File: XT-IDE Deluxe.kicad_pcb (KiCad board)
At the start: 2 copper layers, 100.4 x 96 mm, 58 parts, among them J1 IDE, J10 IRQ5, J11 IRQ7, J2 CF_Adapter, J3 IDE IRQ, J4 VCC, J5 Power Output, J6 MemExp, J7 IRQ2, J8 IRQ3, J9 IRQ4, SW1 HiSpeed, SW2 Config, U1 HCT245, U10 F138, U12 HCT02, U13 AHC1G09, U14 F138, U15 HCT86, U16 F138, U2 HCT573, U3 HCT573, U4 HCT245, U5 HCT04, U6 HCT32, U7 HCT04, U8 28C256, U9 HCT86

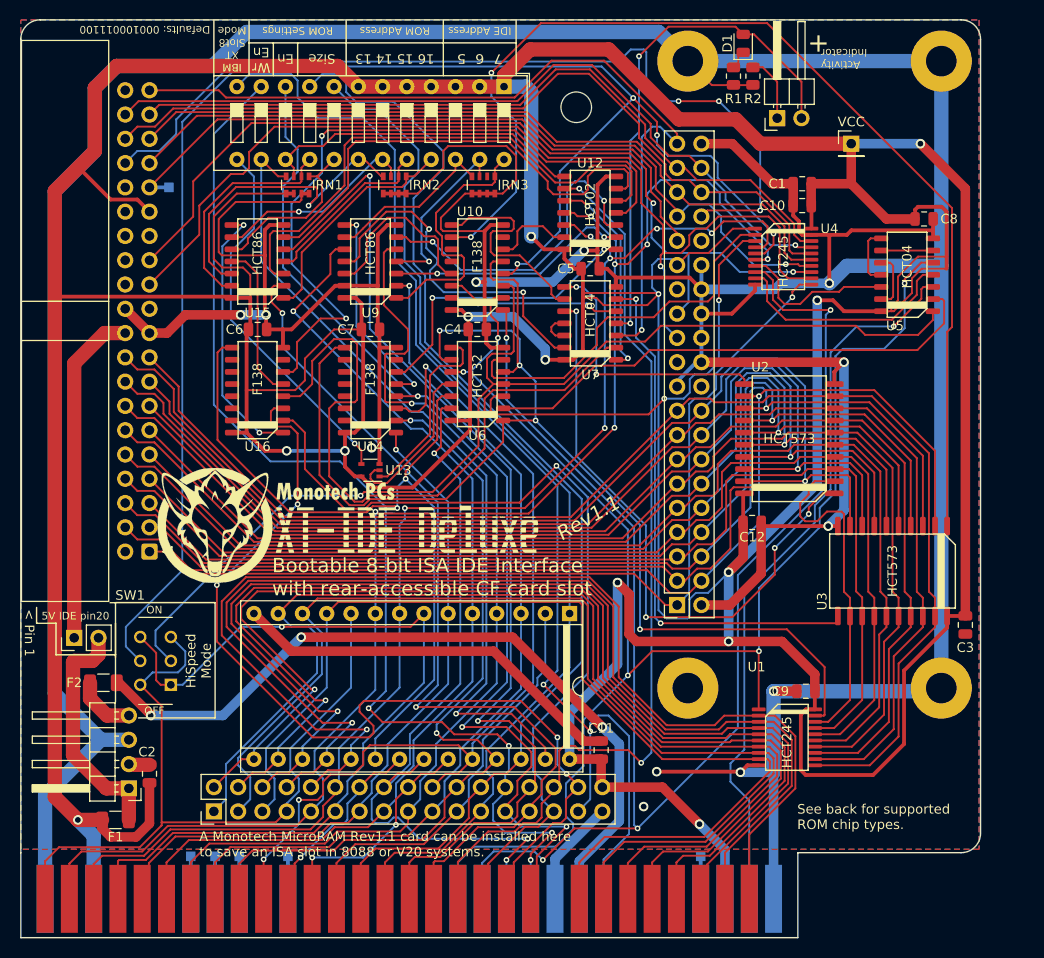
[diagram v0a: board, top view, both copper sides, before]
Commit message: Update to v1.2.
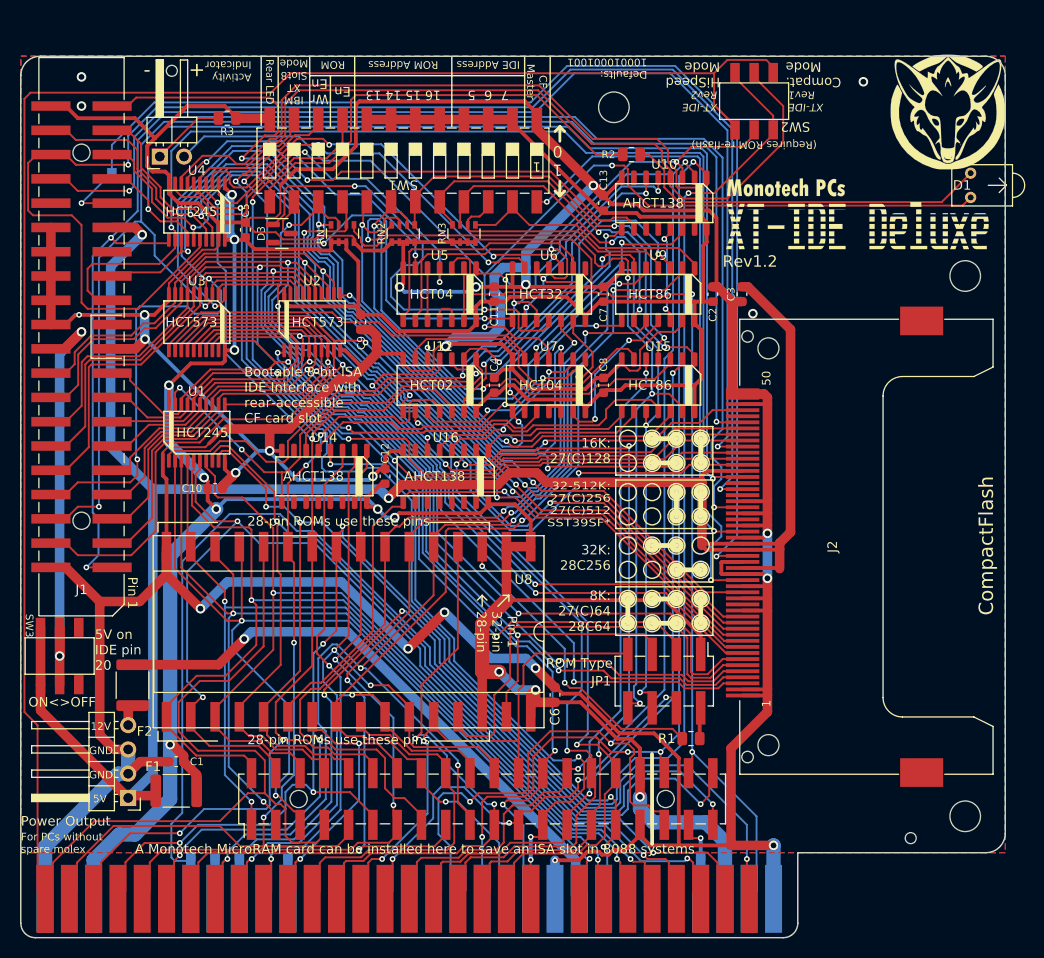
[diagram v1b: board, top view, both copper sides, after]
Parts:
- removed H3, H4: M3, MountingHole:MountingHole_3.2mm_M3_Pad
- removed H5: MountingHole, MountingHole:MountingHole_3.2mm_M3
- removed J4: VCC, Connector_PinHeader_2.54mm:PinHeader_1x01_P2.54mm_Vertical
- removed U13: AHC1G09, Package_TO_SOT_SMD:SOT-353_SC-70-5
- added C13: 100nF, Capacitor_SMD:C_0603_1608Metric, F.Cu at (224.6, 38.6)
- added D3: BAT54A, Package_TO_SOT_SMD:SOT-23, F.Cu at (190.9, 41.8)
- added R3: 220, Resistor_SMD:R_0805_2012Metric, F.Cu at (185.2, 29.7)
- added REF**: JLC_Tooling_Hole, Custom KiCad Library:JLC_Tooling_Hole, F.Cu at (179.4, 24.7)
- added REF**: JLC_Tooling_Hole, Custom KiCad Library:JLC_Tooling_Hole, F.Cu at (256.7, 105.0)
- added SW3: 5V on IDE Pin20, Custom:SW_DPDT_MS-22D28-G020, F.Cu at (167.7, 86.0)
- BUS1: value Bus_ISA_8bit -> 8-bit ISA
- C1, C2: value 106 -> 10uF; footprint Capacitor_SMD:C_0805_2012Metric -> Capacitor_SMD:C_0603_1608Metric
- C10, C11, C12, C3, C4, C5, C6, C7, C8, C9: value 104 -> 100nF; footprint Capacitor_SMD:C_0805_2012Metric -> Capacitor_SMD:C_0603_1608Metric
- D1: value LED -> Rear LED; footprint LED_SMD:LED_0805_2012Metric -> Custom:3mm_LED_RightAngle
- D2: value LED -> LED Header
- F1, F2: footprint Fuse:Fuse_1206_3216Metric -> Fuse:Fuse_1812_4532Metric
- H1, H2: value M3 -> MountingHole; footprint MountingHole:MountingHole_3.2mm_M3_Pad -> MountingHole:MountingHole_3.2mm_M3
- J1: footprint Connector_IDC:IDC-Header_2x20_P2.54mm_Horizontal -> Custom:IDC-20_P2.54mm_Vertical_SMD
- J2: value CF_Adapter -> CF Slot; footprint Connector_PinSocket_2.54mm:PinSocket_2x20_P2.54mm_Vertical -> Custom:CF_Slot_UMax_CFH-R3C1LBMXXMN2
- J6: footprint Connector_PinHeader_2.54mm:PinHeader_2x17_P2.54mm_Vertical -> Custom:MicroRAM_Expansion
- JP1: value 5V IDE pin20 -> ROM Type; footprint Connector_PinHeader_2.54mm:PinHeader_1x02_P2.54mm_Vertical -> Custom:PinHeader_2x04_P2.54mm_Vertical_SMD
- R1, R2: value 1k -> 220
- SW1: value HiSpeed -> Config; footprint Monotech Obscure KiCad Library:SW_MS-22D18G2 -> Button_Switch_SMD:SW_DIP_SPSTx12_Slide_6.7x32.04mm_W8.61mm_P2.54mm_LowProfile
- SW2: value Config -> Rev2; footprint Button_Switch_THT:SW_DIP_SPSTx12_Slide_9.78x32.66mm_W7.62mm_P2.54mm -> Custom:SW_DPDT_MS-22D28-G020
- U10, U14, U16: value F138 -> AHCT138
- U2, U3: footprint Custom KiCad Library:SOIC-20W_7.5x12.8mm_P1.27mm -> Custom KiCad Library:TSSOP-20_4.4x6.5mm_P0.65mm
- U8: value 28C256 -> ROM; footprint Custom KiCad Library:DIP-28_W15.24mm_Socket -> Custom:DIP-32_W16.51mm_SMDSocket_LongPads
- moved C1 89.1 mm to (179.9, 97.0)
- moved LOGO1 88.0 mm to (260.6, 29.1)
- moved H2 84.2 mm to (262.4, 102.7)
- moved C2 77.4 mm to (236.0, 48.1)
- moved U3 77.3 mm to (182.0, 51.0)
- moved U1 69.5 mm to (182.0, 62.6), turned to 90 degrees
- moved R1 69.4 mm to (233.7, 94.6), turned to 0 degrees
- moved C10 68.2 mm to (183.9, 68.4), turned to 0 degrees
- moved D2 64.7 mm to (178.2, 33.7)
- moved JP1 61.9 mm to (230.9, 88.6), turned to -90 degrees
- moved U4 61.5 mm to (182.0, 39.5), turned to -90 degrees
- moved C9 60.5 mm to (199.2, 51.0), turned to -90 degrees
- moved SW1 58.4 mm to (203.6, 34.1), turned to -90 degrees
- moved LOGO2 56.8 mm to (251.3, 39.9)
- moved H1 52.0 mm to (262.4, 46.2)
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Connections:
- net /~{LA1-OE} renamed /~{LA1_OE}
- net /~{LA2-OE} renamed /~{LA2_OE}
- net /~{xLA2-OE} renamed /~{xLA2_OE}
- C3 pad 1: VCC -> /5V_Fused
- F1 pad 1: VCC -> /5V_Fused
- F1 pad 2: /5V_Fused -> VCC
- F2 pad 1: +12V -> /12V_Fused
- F2 pad 2: Net-(F2-Pad2) -> +12V
- J1 pad 20: /IDE_5V -> /IDE_pin20
- J1 pad 21: (no net) -> unconnected-(J1-Pad21)
- J1 pad 27: (no net) -> unconnected-(J1-Pad27)
- J1 pad 29: VCC -> /5V_Fused
- J1 pad 32: (no net) -> unconnected-(J1-Pad32)
- J1 pad 35: /BA0-OR-BA3 -> /B_A0_A3
- J2 pad 1: /~{BRST} -> GND
- J2 pad 10: /DB11 -> GND
- J2 pad 11: /DB3 -> GND
- J2 pad 12: /DB12 -> GND
- J2 pad 13: /DB2 -> /5V_Fused
- J2 pad 14: /DB13 -> GND
- J2 pad 15: /DB1 -> GND
- J2 pad 16: /DB14 -> GND
- J2 pad 17: /DB0 -> GND
- J2 pad 18: /DB15 -> /BA2
- J2 pad 19: GND -> /BA1
- J2 pad 2: GND -> /DB3
- J2 pad 20: (no net) -> /B_A0_A3
- J2 pad 21: (no net) -> /DB0
- J2 pad 22: GND -> /DB1
- J2 pad 23: /~{BIOW} -> /DB2
- J2 pad 24: GND -> unconnected-(J2-Pad24)
- J2 pad 25: /~{BIOR} -> GND
- J2 pad 27: (no net) -> /DB11
- J2 pad 28: GND -> /DB12
- J2 pad 29: VCC -> /DB13
- J2 pad 3: /DB7 -> /DB4
- J2 pad 30: GND -> /DB14
- J2 pad 31: /IDE_IRQ -> /DB15
- J2 pad 32: (no net) -> /~{CS3}
- J2 pad 33: /BA1 -> unconnected-(J2-Pad33)
- J2 pad 34: /~{PDIAG} -> /~{BIOR}
- J2 pad 35: /BA0-OR-BA3 -> /~{BIOW}
- J2 pad 36: /BA2 -> /5V_Fused
- J2 pad 37: /~{CS1} -> /IDE_IRQ
- J2 pad 38: /~{CS3} -> /5V_Fused
- J2 pad 39: /~{DASP} -> /~{Master}
- J2 pad 4: /DB8 -> /DB5
- J2 pad 40: GND -> unconnected-(J2-Pad40)
- J2 pad 6: /DB9 -> /DB7
- J2 pad 7: /DB5 -> /~{CS1}
- J2 pad 8: /DB10 -> GND
- J2 pad 9: /DB4 -> GND
- J5 pad 4: Net-(F2-Pad2) -> /12V_Fused
- JP1 pad 1: /IDE_5V -> VCC
- JP1 pad 2: /5V_Fused -> Net-(JP1-Pad2)
- R1 pad 1: GND -> Net-(R1-Pad1)
- R1 pad 2: Net-(D1-Pad1) -> Net-(JP1-Pad2)
- R2 pad 1: GND -> /~{RearLED_En}
- R2 pad 2: Net-(D2-Pad1) -> Net-(D1-Pad1)
- RN1 pad 1: /ROM_8K_1 -> /Dec_A13
- RN1 pad 2: /ROM_8K_2 -> /~{ROM_EN}
- RN1 pad 3: /~{ROM_EN} -> /~{ROM_WR}
- RN1 pad 4: /~{ROM_WR} -> /~{DASP}
- RN1 pad 7: GND -> VCC
- RN2 pad 1: /ROM_A16 -> /ROM_A15
- RN2 pad 2: /ROM_A15 -> /ROM_A14
- RN2 pad 3: /ROM_A14 -> /ROM_A13
- RN2 pad 4: /ROM_A13 -> /Dec_A14
- RN3 pad 2: (no net) -> /IDE_A6
- RN3 pad 3: /IDE_A6 -> /IDE_A5
- RN3 pad 4: /IDE_A5 -> /ROM_A16
- SW1 pad 1: /A3 -> GND
- SW1 pad 2: /A3-OR-0 -> VCC
- SW1 pad 3: /A0 -> VCC
- SW1 pad 4: /A0 -> VCC
- SW1 pad 5: /A0-OR-3 -> VCC
- SW1 pad 6: /A3 -> VCC
- SW2 pad 1: VCC -> /A3
- SW2 pad 2: VCC -> /A3Compat_A0Speed
- SW2 pad 3: VCC -> /A0
- SW2 pad 4: VCC -> /A0
- SW2 pad 5: VCC -> /A0Compat_A3Speed
- SW2 pad 6: VCC -> /A3
- U1 pad 11: /DB0 -> /DB7
- U1 pad 12: /DB1 -> /DB6
- U1 pad 13: /DB2 -> /DB5
- U1 pad 14: /DB3 -> /DB4
- U1 pad 15: /DB4 -> /DB3
- U1 pad 16: /DB5 -> /DB2
- U1 pad 17: /DB6 -> /DB1
- U1 pad 18: /DB7 -> /DB0
- U1 pad 2: /D7 -> /D0
- U1 pad 3: /D6 -> /D1
- U1 pad 4: /D5 -> /D2
- U1 pad 5: /D4 -> /D3
- U1 pad 6: /D3 -> /D4
- U1 pad 7: /D2 -> /D5
- U1 pad 8: /D1 -> /D6
- U1 pad 9: /D0 -> /D7
- U10 pad 11: (no net) -> unconnected-(U10-Pad11)
- U10 pad 12: (no net) -> unconnected-(U10-Pad12)
- U10 pad 15: (no net) -> unconnected-(U10-Pad15)
- U10 pad 3: /A3-OR-0 -> /A3Compat_A0Speed
- U10 pad 4: /A0-OR-3 -> /A0Compat_A3Speed
- U10 pad 7: (no net) -> unconnected-(U10-Pad7)
- U14 pad 10: (no net) -> unconnected-(U14-Pad10)
- U14 pad 11: (no net) -> unconnected-(U14-Pad11)
- U14 pad 12: (no net) -> unconnected-(U14-Pad12)
- U14 pad 13: (no net) -> unconnected-(U14-Pad13)
- U14 pad 14: (no net) -> unconnected-(U14-Pad14)
- U14 pad 15: (no net) -> unconnected-(U14-Pad15)
- U14 pad 7: (no net) -> unconnected-(U14-Pad7)
- U15 pad 10: /ROM_8K_1 -> /Dec_A14
- U15 pad 13: /ROM_8K_2 -> /Dec_A13
- U16 pad 10: (no net) -> unconnected-(U16-Pad10)
- U16 pad 11: (no net) -> unconnected-(U16-Pad11)
- U16 pad 12: (no net) -> unconnected-(U16-Pad12)
- U16 pad 13: (no net) -> unconnected-(U16-Pad13)
- U16 pad 14: (no net) -> unconnected-(U16-Pad14)
- U16 pad 15: (no net) -> unconnected-(U16-Pad15)
- U16 pad 7: (no net) -> unconnected-(U16-Pad7)
- U2 pad 12: /DB8 -> /DB15
- U2 pad 13: /DB9 -> /DB14
- U2 pad 14: /DB10 -> /DB13
- U2 pad 15: /DB11 -> /DB12
- U2 pad 16: /DB12 -> /DB11
- U2 pad 17: /DB13 -> /DB10
- U2 pad 18: /DB14 -> /DB9
- U2 pad 19: /DB15 -> /DB8
- U2 pad 2: /DB7 -> /DB0
- U2 pad 3: /DB6 -> /DB1
- U2 pad 4: /DB5 -> /DB2
- U2 pad 5: /DB4 -> /DB3
- U2 pad 6: /DB3 -> /DB4
- U2 pad 7: /DB2 -> /DB5
- U2 pad 8: /DB1 -> /DB6
- U2 pad 9: /DB0 -> /DB7
- U4 pad 15: /BA0-OR-BA3 -> /B_A0_A3
- U4 pad 5: /A0-OR-3 -> /A0Compat_A3Speed
- U5 pad 1: /A3-OR-0 -> /~{IOR}
- U5 pad 12: /~{IOR_DELAY} -> Net-(U5-Pad11)
- U5 pad 13: Net-(U5-Pad10) -> Net-(U5-Pad13)
- U5 pad 2: Net-(U5-Pad2) -> Net-(U5-Pad13)
- U5 pad 5: /~{IOR} -> Net-(U5-Pad10)
- U5 pad 6: Net-(U5-Pad6) -> /~{IOR_DELAY}
- U5 pad 8: Net-(U5-Pad11) -> Net-(U5-Pad8)
- U5 pad 9: Net-(U5-Pad6) -> /A3Compat_A0Speed
- U6 pad 2: Net-(U5-Pad2) -> Net-(U5-Pad8)
- U6 pad 4: /A3-OR-0 -> /A3Compat_A0Speed
- U8 pad 1: /A14 -> VCC
- U8 pad 10: /A0 -> /A2
- U8 pad 11: /D0 -> /A1
- U8 pad 12: /D1 -> /A0
- U8 pad 13: /D2 -> /D0
- U8 pad 14: GND -> /D1
- U8 pad 15: /D3 -> /D2
- U8 pad 16: /D4 -> GND
- U8 pad 17: /D5 -> /D3
- U8 pad 18: /D6 -> /D4
- U8 pad 19: /D7 -> /D5
- U8 pad 2: /A12 -> VCC
- U8 pad 20: /~{ROM_CS} -> /D6
- U8 pad 21: /A10 -> /D7
- U8 pad 22: /~{MEMR} -> /~{ROM_CS}
- U8 pad 23: /A11 -> /A10
- U8 pad 24: /A9 -> /~{MEMR}
- U8 pad 25: /A8 -> /A11
- U8 pad 26: /A13 -> /A9
- U8 pad 27: /~{ROM_WR} -> /A8
- U8 pad 28: VCC -> /A13
- U8 pad 3: /A7 -> Net-(R1-Pad1)
- U8 pad 4: /A6 -> /A12
- U8 pad 5: /A5 -> /A7
- U8 pad 6: /A4 -> /A6
- U8 pad 7: /A3 -> /A5
- U8 pad 8: /A2 -> /A4
- U8 pad 9: /A1 -> /A3
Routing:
- net VCC: track 741.4 -> 385.0 mm, vias 13 -> 12
- net /5V_Fused: track 25.1 -> 214.9 mm, vias 0 -> 2
- net /A0: track 80.2 -> 247.2 mm
- net /A0-OR-3: track 161.9 -> 0.00 mm, vias 4 -> 0
- net /A3-OR-0: track 117.1 -> 0.00 mm, vias 1 -> 0
- net /IRQ3: track 4.45 -> 116.0 mm, vias 0 -> 1
- net /A3: track 89.3 -> 192.3 mm, vias 1 -> 5
- net /Dec_A14: track 0.00 -> 101.5 mm, vias 0 -> 3
- net /B_A0_A3: track 0.00 -> 99.9 mm, vias 0 -> 2
- net /Dec_A13: track 0.00 -> 86.3 mm, vias 0 -> 3
- net /IRQ5: track 4.45 -> 89.2 mm, vias 0 -> 3
- net /A0Compat_A3Speed: track 0.00 -> 83.5 mm
- net /BA0-OR-BA3: track 79.1 -> 0.00 mm
- net /BA2: track 85.4 -> 155.8 mm, vias 0 -> 2
- net /A13: track 119.5 -> 53.4 mm, vias 0 -> 2
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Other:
- board size 100.4 x 96 mm -> 103 x 92.2 mm
- board text added: "(Requires ROM re-flash)"
- board text added: "+12V"
- board text added: "+5V"
- board text added: "1 0"
- board text added: "12V"
- board text added: "16K: 27(C)128"
- board text added: "234 IDE 000 300 <Default 001 320 010 340 011 360 100 380 101 3A0 110 3C0 111 3E0"
- board text added: "28-pin ROMs use these pins"
- board text added: "32-512K: 27(C)256 27(C)512 SST39SF*"
- board text added: "32K: 28C256"
- board text added: "5678 ROM 0000 C0000* 0001 C2000 0010 C4000- 0011 C6000 0100 C8000* 0101 CA000 0110 CC000- 0111 CE000 1000 D0000* <Default 1001 D2000 1010 D4000- 1011 D6000 1100 D8000* 1101 DA000 1110 DC000- 1111 DE000"
- board text added: "5V"
- board text added: "5V on IDE pin 20"
- board text added: "8K: 27(C)64 28C64"
- board text added: "= All ROMs supported = 16K or 8K ROMs only = 8K ROMs only"
- board text added: "= Controller Type: XT-IDE Rev1 = Controller Type: XT-IDE Rev2"
- board text added: "A Monotech MicroRAM card can be installed here to save an ISA slot in 8088 systems"
- board text added: "CF Master"
- board text added: "Compat. Mode"
- board text added: "Defaults: 100010001001"
- board text added: "Disable the Boot ROM by turning OFF config switch 9 if your settings cause inability to boot. Turn ON while system is running to re-flash from DOS."
- board text added: "Ensure XT-IDE BIOS is positioned above any other boot ROMs in the system, or it will only allow using the drives, but not booting from them. Write-disable the ROM by turning OFF switch 10 once the system is up and running the way intended, to prevent accidental re-flashing. Changing IDE Address requires re-configuring and re-flashing XT-IDE BIOS. Changing ROM Address doesn't require any other cha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"
- board text added: "For PCs without spare molex"
- board text added: "GND"
- board text added: "IDE Pin 1"
- board text added: "MONOTECH PCs - 2023 XT-IDE DELUXE Rev1.2"
- board text added: "ON<>OFF"
- board text added: "Pin 1"
- board text added: "Pin 1 32-pin 28-pin"
- board text added: "Power Output"
- board text added: "ROM"
- board text added: "Rear LED"
- board text added: "Rev1.2"
- board text added: "XT-IDE Rev1"
- board text added: "XT-IDE Rev2"
- board text removed: "+12V GND +5V"
- board text removed: "123 IDE 000 300 <Default 001 320 010 340 011 360 100 380 101 3A0 110 3C0 111 3E0"
- board text removed: "28C64 / 2764 / 27C64 27128 / 27C128 28C256 (not 27(C)256)"
- board text removed: "4567 ROM 0000 C0000* 0001 C2000 0010 C4000- 0011 C6000 0100 C8000* 0101 CA000 0110 CC000- 0111 CE000 1000 D0000* <Default 1001 D2000 1010 D4000- 1011 D6000 1100 D8000* 1101 DA000 1110 DC000- 1111 DE000"
- board text removed: "89 ROM Size 11 8K 10 16K 00 32K"
- board text removed: "8K 16K 32K"
- board text removed: "< Pin 1"
- board text removed: "= All ROMs support = 16K/8K ROM support = 8K ROM support"
- board text removed: "A Monotech MicroRAM Rev1.1 card can be installed here to save an ISA slot in 8088 or V20 systems."
- board text removed: "Based on the XT-IDE Rev2 of VCFed Forum, and XT-IDE Rev4 of GlitchWorks: github.com/glitchwrks/xt_ide Uses XT-IDE Universal BIOS: xtideuniversalbios.org"
- board text removed: "Defaults: 000100011100"
- board text removed: "Disable the Boot ROM by turning OFF switch 10 if your settings cause inability to boot. Turn ON while system is running to re-flash from DOS. Ensure XT-IDE BIOS is positioned above any other boot ROMs in the system, or it will only allow using the drives, but not booting them. Changing IDE Address requires re-configuring and re-flashing XT-IDE BIOS with XTIDECFG. Changing ROM Address doesn't requ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"
- board text removed: "MONOTECH PCs - 2020 XT-IDE DELUXE Rev1.1"
- board text removed: "OFF"
- board text removed: "ON"
- board text removed: "Only 28C64 and 28C256 can be written to."
- board text removed: "ROM Chips Supported"
- board text removed: "ROM Settings"
- board text removed: "ROM Size Switches"
- board text removed: "Rev1.1"
- board text removed: "See back for supported ROM chip types."
- board text removed: "Size"
- board text removed: "Write-disable the ROM by turning OFF switch 11 once the system is up and running the way intended, to prevent accidental re-flashing."
